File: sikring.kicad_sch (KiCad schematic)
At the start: 7 parts, among them IC1 TPS259830LNRGER, IC2 TPS259830LNRGER, IC3 TPS259830LNRGER

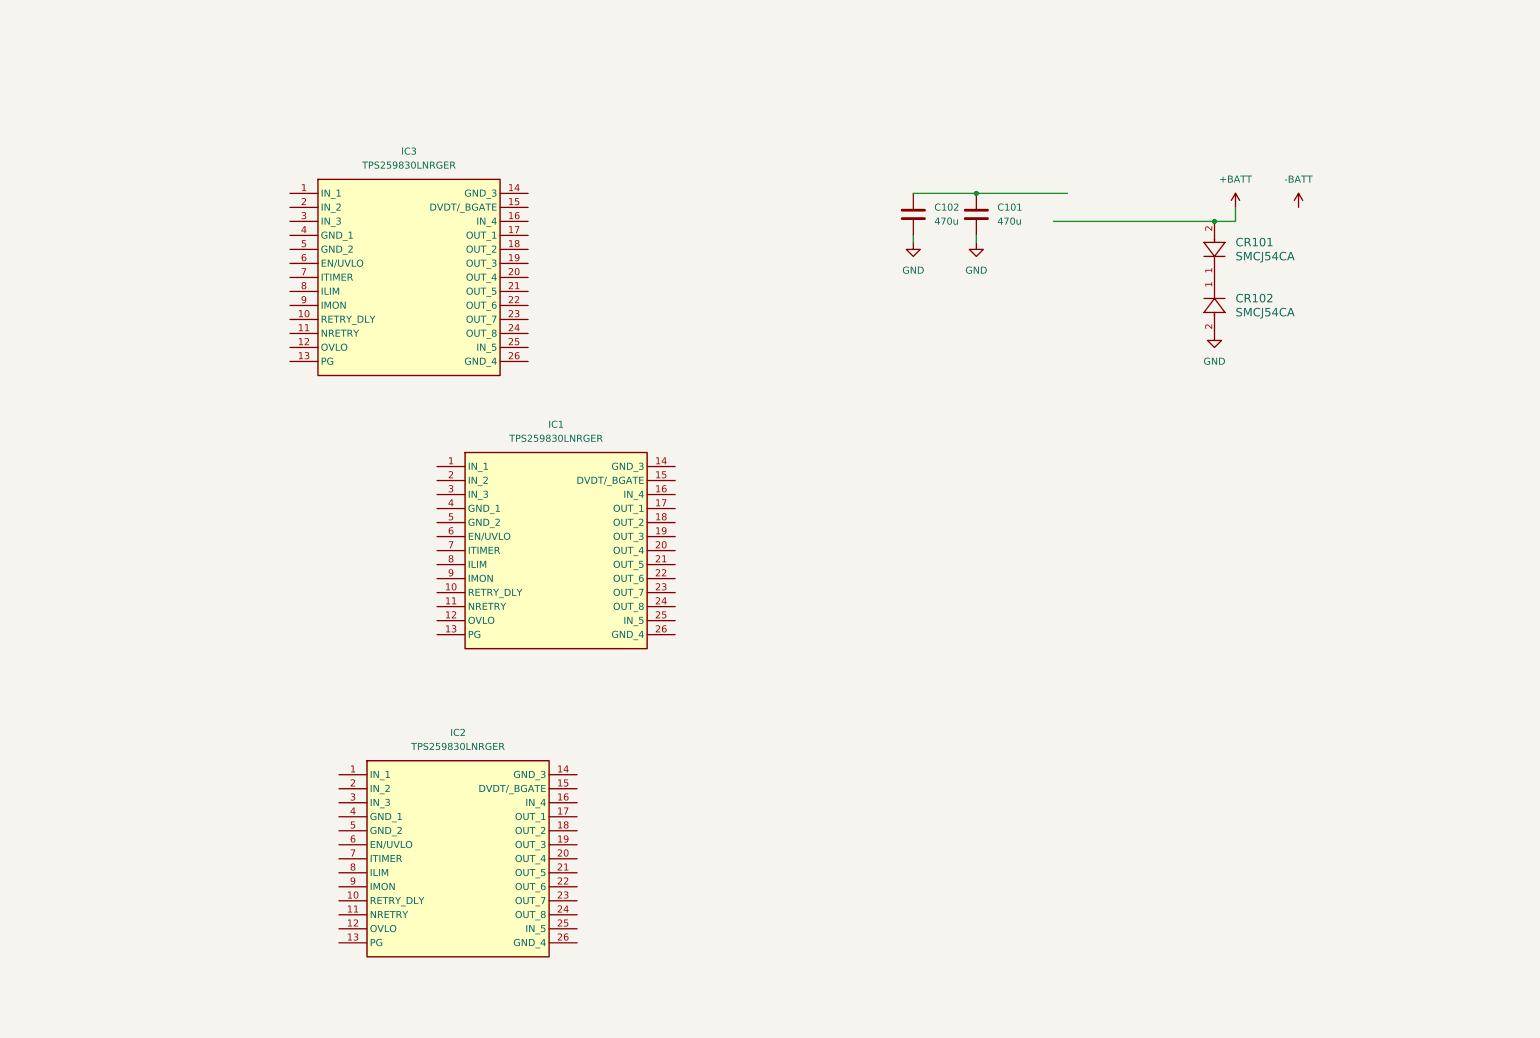
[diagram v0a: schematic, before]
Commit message: lagt inn alle ideele komp mangler å finne faktiske komponenter
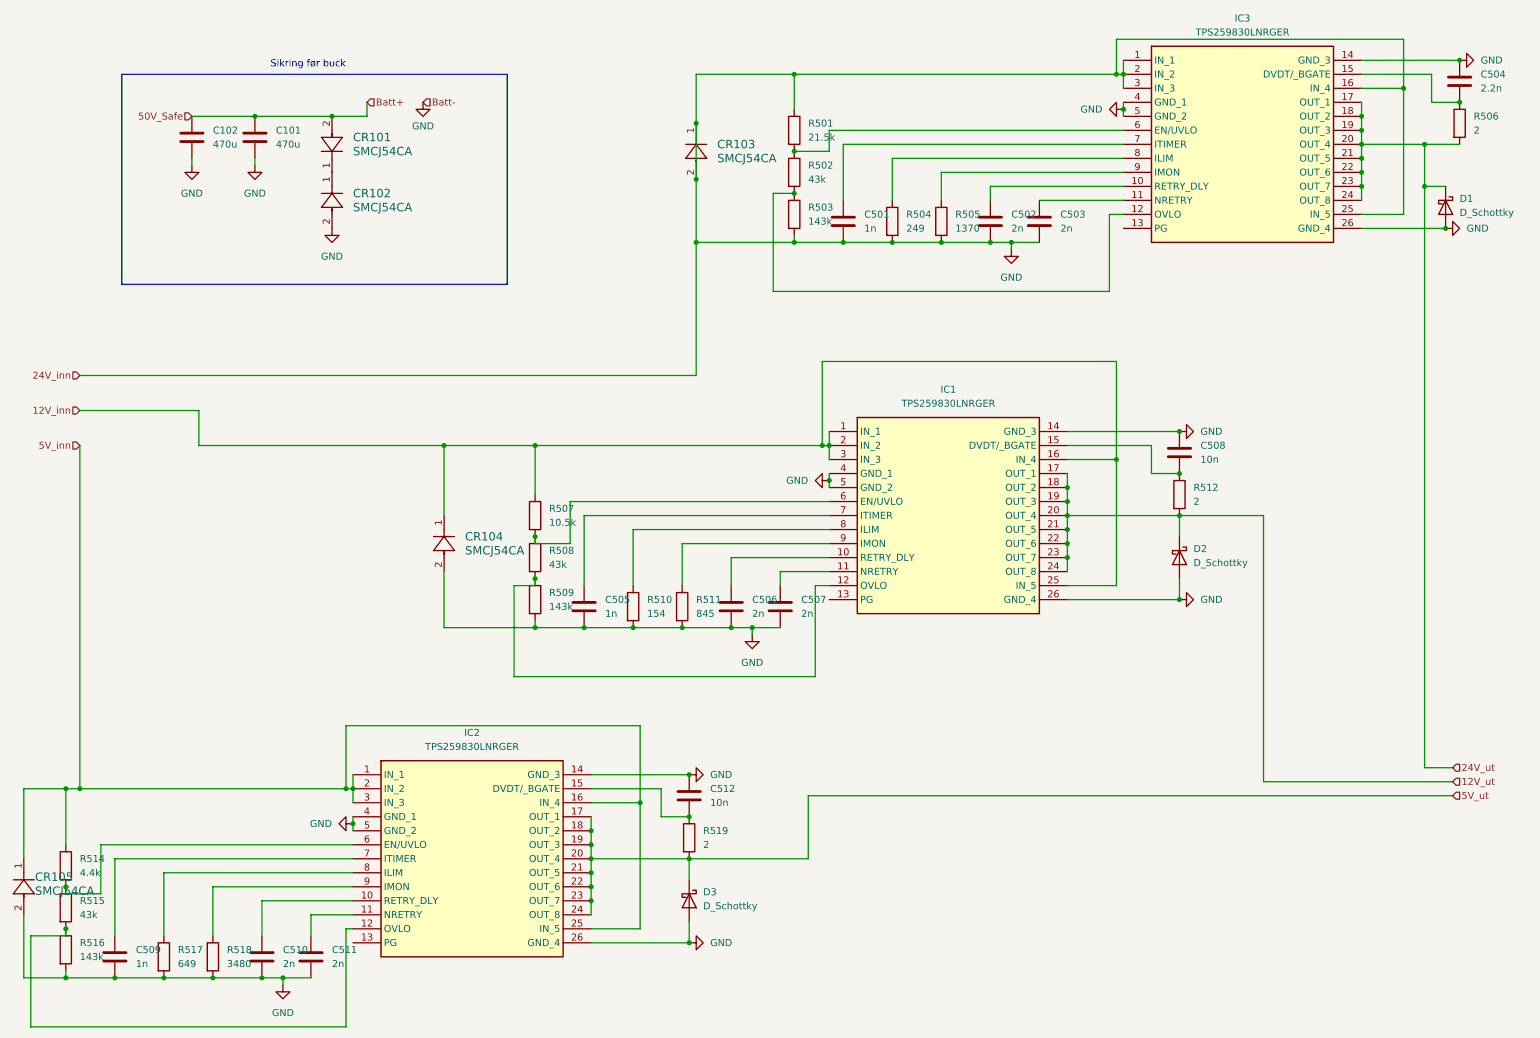
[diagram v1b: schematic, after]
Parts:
- added C501, C505, C509: 1n, symbol Device:C
- added C502, C503, C506, C507, C510, C511: 2n, symbol Device:C
- added C504: 2.2n, symbol Device:C
- added C508, C512: 10n, symbol Device:C
- added CR103, CR104, CR105: SMCJ54CA, SMCJSeries_LTF, symbol Halfdan:SMCJ54CA
- added D1, D2, D3: D_Schottky, Package_SON:WSON-8-1EP_6x5mm_P1.27mm_EP3.4x4mm, symbol Device:D_Schottky
- added R501: 21.5k, CAPAE830X1000N, symbol Device:R
- added R502, R508, R515: 43k, CAPAE830X1000N, symbol Device:R
- added R503, R509, R516: 143k, CAPAE830X1000N, symbol Device:R
- added R504: 249, CAPAE830X1000N, symbol Device:R
- added R505: 1370, CAPAE830X1000N, symbol Device:R
- added R506, R512, R519: 2, symbol Device:R
- added R507: 10.5k, CAPAE830X1000N, symbol Device:R
- added R510: 154, CAPAE830X1000N, symbol Device:R
- added R511: 845, CAPAE830X1000N, symbol Device:R
- added R514: 4.4k, CAPAE830X1000N, symbol Device:R
- added R517: 649, CAPAE830X1000N, symbol Device:R
- added R518: 3480, CAPAE830X1000N, symbol Device:R
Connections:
- net +BATT is gone; now on net 50V_Safe: CR101.2
- net GND: now also IC1.14 (GND_3), IC1.26 (GND_4), IC1.4 (GND_1), IC1.5 (GND_2), IC2.14 (GND_3), IC2.26 (GND_4), IC2.4 (GND_1), IC2.5 (GND_2), IC3.1 (IN_1), IC3.14 (GND_3), IC3.16 (IN_4), IC3.2 (IN_2), IC3.25 (IN_5), IC3.26 (GND_4), IC3.3 (IN_3), IC3.4 (GND_1), IC3.5 (GND_2), C501.2, C502.2, C503.2, C504.1, C505.2, C506.2, C507.2, C508.1, C509.2, C510.2, C511.2, C512.1, CR103.1, CR103.2, CR104.2, CR105.2, D1.2 (A), D2.2 (A), D3.2 (A), R501.1, R503.2, R504.2, R505.2, R509.2, R510.2, R511.2, R516.2, R517.2, R518.2
- net 50V_Safe: now reaches C101.2, C102.1
- net 5V_inn: now reaches IC2.1 (IN_1)
- net 5V_inn: now also IC2.16 (IN_4), IC2.2 (IN_2), IC2.25 (IN_5), IC2.3 (IN_3), CR105.1, R514.1
- net at IC2.10 (RETRY_DLY): now also C510.1
- net at IC2.11 (NRETRY): now also C511.1
- net at IC2.12 (OVLO): now also R515.2, R516.1
- net at IC2.15 (DVDT/_BGATE): now also C512.2, R519.1
- net 5V_ut: now reaches IC2.17 (OUT_1)
- net 5V_ut: now also IC2.18 (OUT_2), IC2.19 (OUT_3), IC2.20 (OUT_4), IC2.21 (OUT_5), IC2.22 (OUT_6), IC2.23 (OUT_7), IC2.24 (OUT_8), D3.1 (K), R519.2
- net at IC2.6 (EN/UVLO): now also R514.2, R515.1
- net at IC2.7 (ITIMER): now also C509.1
- net at IC2.8 (ILIM): now also R517.1
- net at IC2.9 (IMON): now also R518.1
- net at IC3.10 (RETRY_DLY): now also C502.1
- net at IC3.11 (NRETRY): now also C503.1
- net at IC3.12 (OVLO): now also R502.2, R503.1
- net at IC3.15 (DVDT/_BGATE): now also C504.2, R506.1
- net 24V_ut: now reaches IC3.17 (OUT_1)
- net 24V_ut: now also IC3.18 (OUT_2), IC3.19 (OUT_3), IC3.20 (OUT_4), IC3.21 (OUT_5), IC3.22 (OUT_6), IC3.23 (OUT_7), IC3.24 (OUT_8), D1.1 (K), R506.2
- net at IC3.6 (EN/UVLO): now also R501.2, R502.1
- net at IC3.7 (ITIMER): now also C501.1
- net at IC3.8 (ILIM): now also R504.1
- net at IC3.9 (IMON): now also R505.1
- net 12V_inn: now reaches IC1.1 (IN_1)
- net 12V_inn: now also IC1.16 (IN_4), IC1.2 (IN_2), IC1.25 (IN_5), IC1.3 (IN_3), CR104.1, R507.1
- net at IC1.10 (RETRY_DLY): now also C506.1
- net at IC1.11 (NRETRY): now also C507.1
- net at IC1.12 (OVLO): now also R508.2, R509.1
- net at IC1.15 (DVDT/_BGATE): now also C508.2, R512.1
- net 12V_ut: now reaches IC1.17 (OUT_1)
- net 12V_ut: now also IC1.18 (OUT_2), IC1.19 (OUT_3), IC1.20 (OUT_4), IC1.21 (OUT_5), IC1.22 (OUT_6), IC1.23 (OUT_7), IC1.24 (OUT_8), D2.1 (K), R512.2
- net at IC1.6 (EN/UVLO): now also R507.2, R508.1
- net at IC1.7 (ITIMER): now also C505.1
- net at IC1.8 (ILIM): now also R510.1
- net at IC1.9 (IMON): now also R511.1
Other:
- note added: "Sikring før buck"
- moved on the sheet: IC1, IC2, IC3
